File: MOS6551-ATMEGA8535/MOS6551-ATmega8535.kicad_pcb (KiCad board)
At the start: 2 copper layers, 19.8 x 41.8 mm, 8 parts, among them J1 Conn_02x03_Odd_Even, J2 Conn_02x14_Counter_Clockwise, U1 ATmega8535-16AU, Y1 Crystal

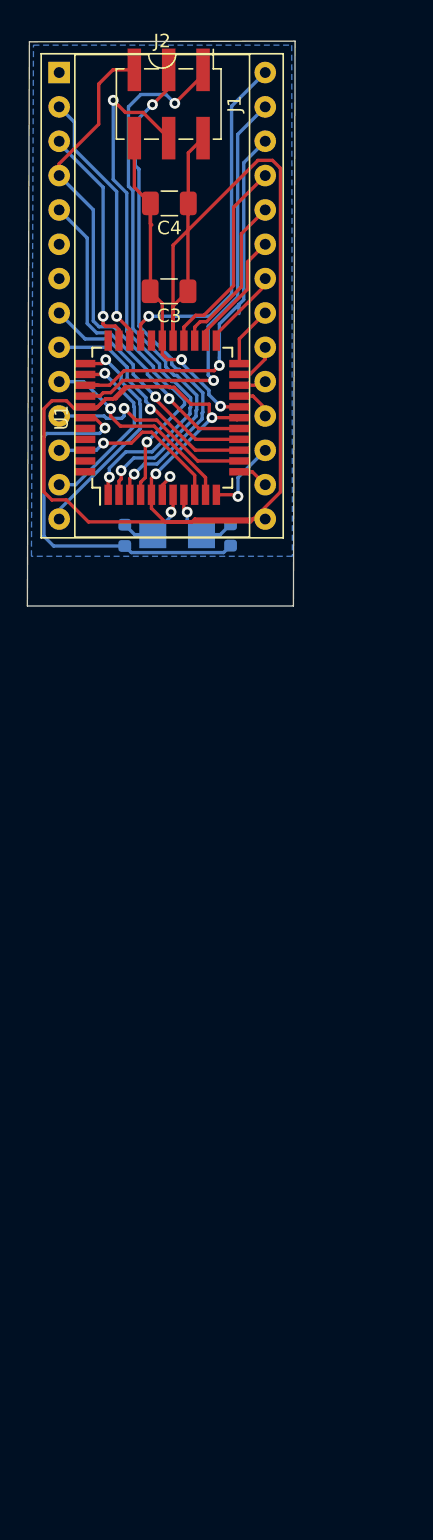
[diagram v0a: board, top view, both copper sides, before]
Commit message: Another darft
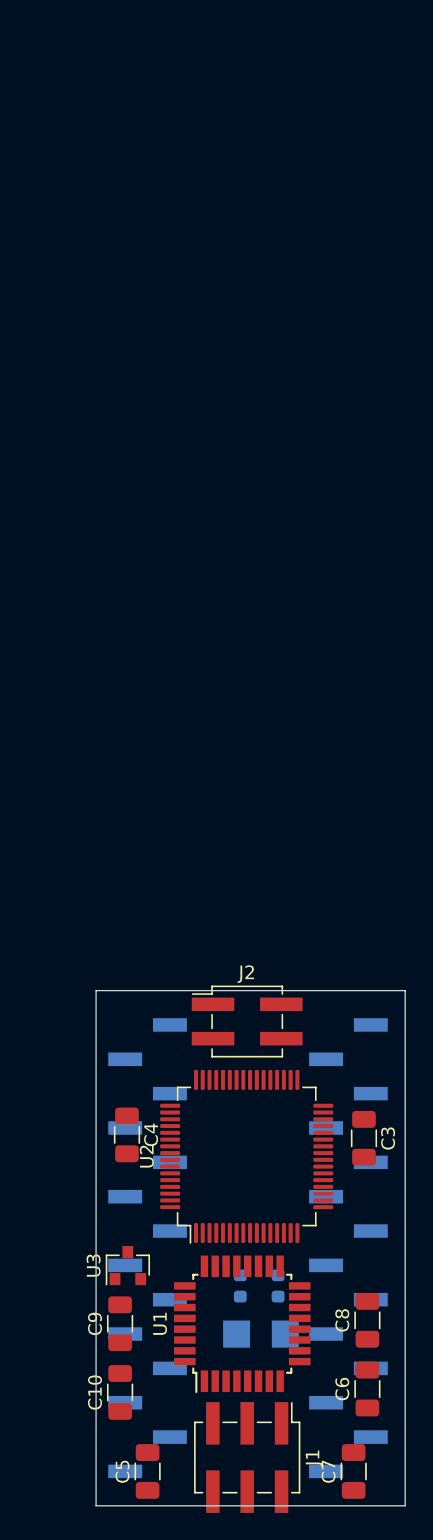
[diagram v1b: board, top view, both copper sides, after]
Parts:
- added C10: 1nF, Capacitor_SMD:C_1206_3216Metric, F.Cu at (140.2, 170.7)
- added C5: 1µF, Capacitor_SMD:C_1206_3216Metric, F.Cu at (142.2, 176.5)
- added C6: 1nF, Capacitor_SMD:C_1206_3216Metric, F.Cu at (158.5, 170.4)
- added C7: 1µF, Capacitor_SMD:C_1206_3216Metric, F.Cu at (157.5, 176.5)
- added C8: 1nF, Capacitor_SMD:C_1206_3216Metric, F.Cu at (158.5, 165.4)
- added C9: 1µF, Capacitor_SMD:C_1206_3216Metric, F.Cu at (140.2, 165.6)
- added J3: Conn_01x14, Connector_PinHeader_2.54mm:PinHeader_1x14_P2.54mm_Vertical_SMD_Pin1Left, B.Cu at (142.2, 160.0)
- added J4: Conn_01x14, Connector_PinHeader_2.54mm:PinHeader_1x14_P2.54mm_Vertical_SMD_Pin1Left, B.Cu at (157.1, 160.0)
- added U2: XC9572XL-VQ64, Package_QFP:TQFP-64_10x10mm_P0.5mm, F.Cu at (149.6, 153.2)
- added U3: MCP1700-3302E_SOT23, Package_TO_SOT_SMD:SOT-23, F.Cu at (140.8, 161.3)
- J2: value Conn_02x14_Counter_Clockwise -> Conn_02x02_Counter_Clockwise; footprint Package_DIP:DIP-28_W15.24mm_Socket -> Connector_PinHeader_2.54mm:PinHeader_2x02_P2.54mm_Vertical_SMD
- U1: value ATmega8535-16AU -> ATmega88-20AU; footprint Package_QFP:TQFP-44_10x10mm_P0.8mm -> Package_QFP:TQFP-32_7x7mm_P0.8mm
- moved J1 100.3 mm to (149.6, 175.5)
- moved J2 71.5 mm to (149.6, 143.3)
- moved C4 69.0 mm to (140.7, 151.6), turned to 270 degrees
- moved U1 67.3 mm to (149.2, 165.6)
- moved C3 64.3 mm to (158.2, 151.9), turned to 270 degrees
- moved Y1 59.4 mm to (150.6, 166.4)
- moved C2 56.2 mm to (149.1, 162.8), turned to 270 degrees
- moved C1 55.7 mm to (151.9, 162.8), turned to 270 degrees
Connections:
- J2 pad 1: GND -> Net-(J2-Pad1)
- J2 pad 2: CS0 -> Net-(J2-Pad2)
- J2 pad 3: ~CS1 -> Net-(J2-Pad3)
- J2 pad 4: ~RESET -> Net-(J2-Pad4)
- U1 pad 1: MOSI -> ~DCD
- U1 pad 10: TxD -> ~RTS
- U1 pad 11: ~DSR -> RxC
- U1 pad 12: ~DCD -> Net-(U1-Pad12)
- U1 pad 13: ~DTR -> Net-(U1-Pad13)
- U1 pad 14: ~CTS -> SCK
- U1 pad 15: ~RTS -> MOSI
- U1 pad 16: RxC -> MISO
- U1 pad 17: +5V -> Net-(U1-Pad17)
- U1 pad 18: GND -> +5V
- U1 pad 19: DB0 -> (no net)
- U1 pad 2: MISO -> ~DTR
- U1 pad 20: DB1 -> (no net)
- U1 pad 21: DB2 -> GND
- U1 pad 22: DB3 -> (no net)
- U1 pad 23: DB4 -> Net-(U1-Pad23)
- U1 pad 24: DB5 -> Net-(U1-Pad24)
- U1 pad 25: DB6 -> Net-(U1-Pad25)
- U1 pad 26: DB7 -> Net-(U1-Pad26)
- U1 pad 27: +5V -> Net-(U1-Pad27)
- U1 pad 28: GND -> Net-(U1-Pad28)
- U1 pad 29: (no net) -> ~RESET
- U1 pad 3: SCK -> GND
- U1 pad 30: R~W -> RxD
- U1 pad 31: CS0 -> TxD
- U1 pad 32: ~CS1 -> ~DSR
- U1 pad 4: ~RESET -> +5V
- U1 pad 5: +5V -> GND
- U1 pad 6: GND -> +5V
- U1 pad 9: RxD -> ~CTS
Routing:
- net +5V: track 125.6 -> 0.00 mm, vias 2 -> 0
- net GND: track 57.4 -> 0.00 mm, vias 4 -> 0
- net MISO: track 41.6 -> 0.00 mm, vias 2 -> 0
- net ~RESET: track 40.6 -> 0.00 mm, vias 1 -> 0
- net MOSI: track 40.6 -> 0.00 mm, vias 2 -> 0
- net SCK: track 39.6 -> 0.00 mm, vias 2 -> 0
- net CLK: track 32.1 -> 0.00 mm, vias 1 -> 0
- net ~IRQ: track 30.3 -> 0.00 mm, vias 1 -> 0
- net R~W: track 26.3 -> 0.00 mm, vias 1 -> 0
- net RxC: track 24.0 -> 0.00 mm, vias 1 -> 0
- net CS0: track 19.4 -> 0.00 mm, vias 1 -> 0
- net ~RTS: track 17.7 -> 0.00 mm, vias 1 -> 0
- net ~CTS: track 17.3 -> 0.00 mm, vias 1 -> 0
- net ~CS1: track 17.0 -> 0.00 mm, vias 1 -> 0
- net RS1: track 17.0 -> 0.00 mm, vias 1 -> 0
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- removed copper zone on B.Cu, net GND
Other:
- board size 19.8 x 41.8 mm -> 22.9 x 38.1 mm
